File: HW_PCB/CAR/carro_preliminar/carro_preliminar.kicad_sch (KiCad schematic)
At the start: 44 parts, among them IC1 TB6612FNG, J1 V_Battery, J2 STLINK, J3 Motores, J4 BATTLEDS, J5 UART, J6 Servo_Motor, J7 NRF24L01, SW1 SW_DPST_x2, U1 STM32F103C8Tx, U2 AMS1117-3.3, U3 AMS1117-3.3, U5 AMS1117-5.0, Y1 8MHz

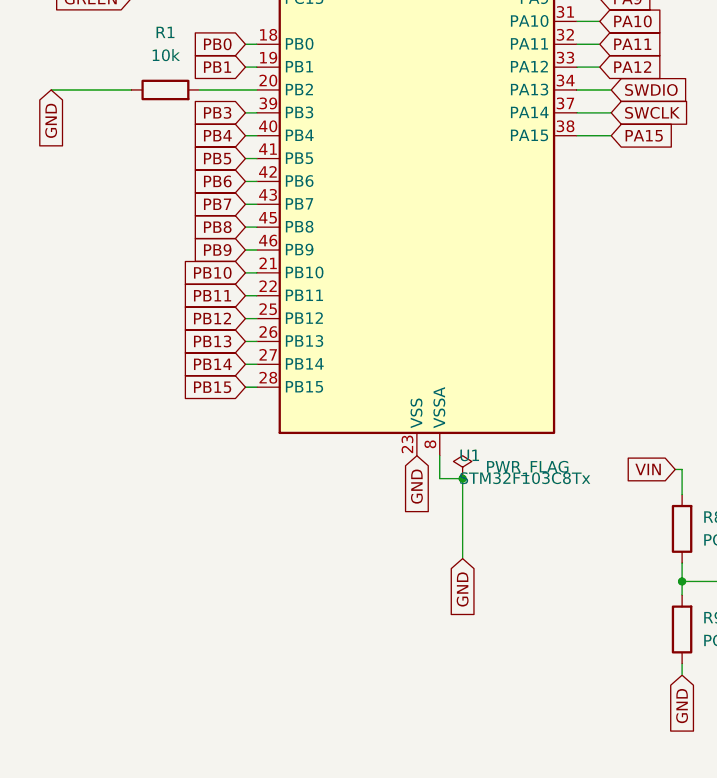
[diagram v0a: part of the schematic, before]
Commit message: PCBCAR FULL
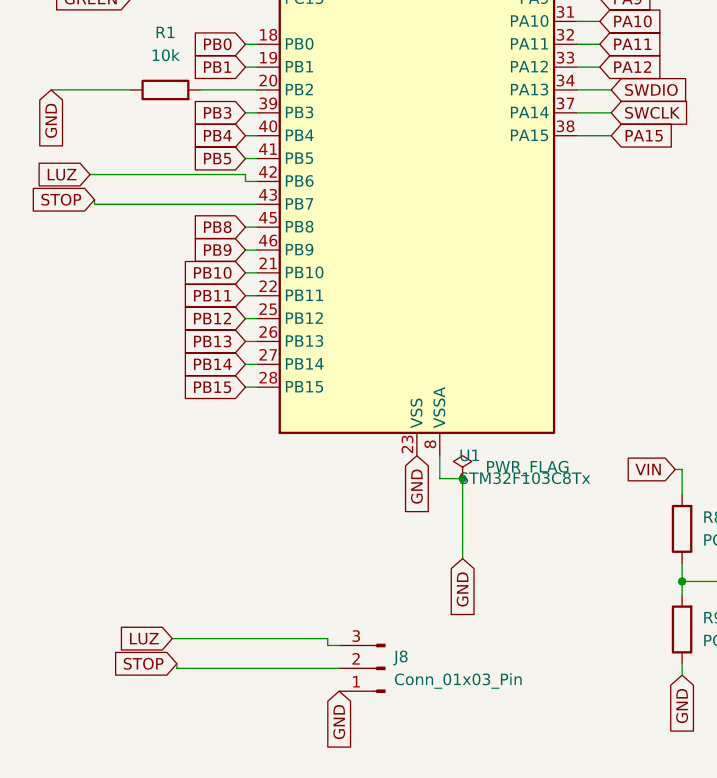
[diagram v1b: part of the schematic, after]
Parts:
- added J8: Conn_01x03_Pin, Connector_PinHeader_2.54mm:PinHeader_1x03_P2.54mm_Vertical, symbol Connector:Conn_01x03_Pin
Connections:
- net GND: now also J8.1 (Pin_1)
- net PB6 renamed LUZ
- net LUZ: now also J8.3 (Pin_3)
- net PB7 renamed STOP
- net STOP: now also J8.2 (Pin_2)
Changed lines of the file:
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@@
 	(wire
 		(pts
+			(xy 47.244 184.15) (xy 47.244 184.912)
+		)
+		(stroke
+			(width 0)
+			(type default)
+		)
+	)
+	(wire
+		(pts
 			(xy 161.29 71.12) (xy 161.29 90.17)
 		)
@@
 	(wire
 		(pts
-			(xy 38.1 135.89) (xy 39.37 135.89)
-		)
-		(stroke
-			(width 0)
-			(type default)
-		)
-	)
-	(wire
-		(pts
 			(xy 161.29 119.38) (xy 162.56 119.38)
 		)
@@
 	(wire
 		(pts
+			(xy 21.336 135.382) (xy 21.336 135.89)
+		)
+		(stroke
+			(width 0)
+			(type default)
+		)
+	)
+	(wire
+		(pts
 			(xy 229.108 138.684) (xy 242.062 138.684)
 		)
@@
 	(wire
 		(pts
+			(xy 20.828 132.588) (xy 38.1 132.588)
+		)
+		(stroke
+			(width 0)
+			(type default)
+		)
+	)
+	(wire
+		(pts
 			(xy 74.93 107.95) (xy 77.47 107.95)
 		)
@@
 	(wire
 		(pts
+			(xy 29.972 184.15) (xy 47.244 184.15)
+		)
+		(stroke
+			(width 0)
+			(type default)
+		)
+	)
+	(wire
+		(pts
 			(xy 38.1 133.35) (xy 39.37 133.35)
 		)
@@
 	(wire
 		(pts
+			(xy 21.336 135.89) (xy 39.37 135.89)
+		)
+		(stroke
+			(width 0)
+			(type default)
+		)
+	)
+	(wire
+		(pts
 			(xy 172.72 77.47) (xy 175.26 77.47)
 		)
@@
 	(wire
 		(pts
+			(xy 38.1 132.588) (xy 38.1 133.35)
+		)
+		(stroke
+			(width 0)
+			(type default)
+		)
+	)
+	(wire
+		(pts
 			(xy 91.694 177.8) (xy 86.614 177.8)
 		)
@@
 	(wire
 		(pts
+			(xy 30.48 187.452) (xy 48.514 187.452)
+		)
+		(stroke
+			(width 0)
+			(type default)
+		)
+	)
+	(wire
+		(pts
 			(xy 214.63 74.93) (xy 214.63 97.79)
 		)
@@
 	(wire
 		(pts
+			(xy 30.48 186.944) (xy 30.48 187.452)
+		)
+		(stroke
+			(width 0)
+			(type default)
+		)
+	)
+	(wire
+		(pts
 			(xy 191.262 147.32) (xy 191.262 152.908)
 		)
@@
 	(wire
 		(pts
+			(xy 47.244 184.912) (xy 48.514 184.912)
+		)
+		(stroke
+			(width 0)
+			(type default)
+		)
+	)
+	(wire
+		(pts
 			(xy 57.15 78.74) (xy 57.15 82.55)
 		)
@@
 		)
 	)
+	(global_label "GND"
+		(shape input)
+		(at 48.514 189.992 270)
+		(fields_autoplaced yes)
+		(effects
+			(font
+				(size 1.27 1.27)
+			)
+			(justify right)
+		)
+		(property "Intersheetrefs" "${INTERSHEET_REFS}"
+			(at 48.514 196.8477 90)
+			(effects
+				(font
+					(size 1.27 1.27)
+				)
+				(justify right)
+				(hide yes)
+			)
+		)
+	)
 	(global_label "PA6"
 		(shape input)
@@
 		)
 	)
+	(global_label "STOP"
+		(shape input)
+		(at 21.336 135.382 180)
+		(fields_autoplaced yes)
+		(effects
+			(font
+				(size 1.27 1.27)
+			)
+			(justify right)
+		)
+		(property "Intersheetrefs" "${INTERSHEET_REFS}"
+			(at 13.5732 135.382 0)
+			(effects
+				(font
+					(size 1.27 1.27)
+				)
+				(justify right)
+				(hide yes)
+			)
+		)
+	)
 	(global_label "GND"
 		(shape input)
@@
 		)
 	)
-	(global_label "PB7"
-		(shape input)
-		(at 38.1 135.89 180)
-		(fields_autoplaced yes)
-		(effects
-			(font
-				(size 1.27 1.27)
-			)
-			(justify right)
-		)
-		(property "Intersheetrefs" "${INTERSHEET_REFS}"
-			(at 31.3653 135.89 0)
-			(effects
-				(font
-					(size 1.27 1.27)
-				)
-				(justify right)
-				(hide yes)
-			)
-		)
-	)
 	(global_label "GND"
 		(shape input)
@@
 		)
 	)
+	(global_label "STOP"
+		(shape input)
+		(at 30.48 186.944 180)
+		(fields_autoplaced yes)
+		(effects
+			(font
+				(size 1.27 1.27)
+			)
+			(justify right)
+		)
+		(property "Intersheetrefs" "${INTERSHEET_REFS}"
+			(at 22.7172 186.944 0)
+			(effects
+				(font
+					(size 1.27 1.27)
+				)
+				(justify right)
+				(hide yes)
+			)
+		)
+	)
 	(global_label "PA0"
 		(shape input)
@@
 		)
 	)
+	(global_label "LUZ"
+		(shape input)
+		(at 29.972 184.15 180)
+		(fields_autoplaced yes)
+		(effects
+			(font
+				(size 1.27 1.27)
+			)
+			(justify right)
+		)
+		(property "Intersheetrefs" "${INTERSHEET_REFS}"
+			(at 23.4187 184.15 0)
+			(effects
+				(font
+					(size 1.27 1.27)
+				)
+				(justify right)
+				(hide yes)
+			)
+		)
+	)
 	(global_label "GREEN"
 		(shape input)
@@
 		)
 	)
-	(global_label "PB6"
-		(shape input)
-		(at 38.1 133.35 180)
-		(fields_autoplaced yes)
-		(effects
-			(font
-				(size 1.27 1.27)
-			)
-			(justify right)
-		)
-		(property "Intersheetrefs" "${INTERSHEET_REFS}"
-			(at 31.3653 133.35 0)
-			(effects
-				(font
-					(size 1.27 1.27)
-				)
-				(justify right)
-				(hide yes)
-			)
-		)
-	)
 	(global_label "PB0"
 		(shape input)
@@
 		)
 	)
+	(global_label "LUZ"
+		(shape input)
+		(at 20.828 132.588 180)
+		(fields_autoplaced yes)
+		(effects
+			(font
+				(size 1.27 1.27)
+			)
+			(justify right)
+		)
+		(property "Intersheetrefs" "${INTERSHEET_REFS}"
+			(at 14.2747 132.588 0)
+			(effects
+				(font
+					(size 1.27 1.27)
+				)
+				(justify right)
+				(hide yes)
+			)
+		)
+	)
 	(global_label "VCC"
 		(shape input)
@@
 					(unit 1)
 				)
+			)
+		)
+	)
+	(symbol
+		(lib_id "Connector:Conn_01x03_Pin")
+		(at 53.594 187.452 180)
+		(unit 1)
+		(exclude_from_sim no)
+		(in_bom yes)
+		(on_board yes)
+		(dnp no)
+		(fields_autoplaced yes)
+		(property "Reference" "J8"
+			(at 54.61 186.1819 0)
+			(effects
+				(font
+					(size 1.27 1.27)
+				)
+				(justify right)
+			)
+		)
+		(property "Value" "Conn_01x03_Pin"
+			(at 54.61 188.7219 0)
+			(effects
+				(font
+					(size 1.27 1.27)
+				)
+				(justify right)
+			)
+		)
+		(property "Footprint" "Connector_PinHeader_2.54mm:PinHeader_1x03_P2.54mm_Vertical"
+			(at 53.594 187.452 0)
+			(effects
+				(font
+					(size 1.27 1.27)
+				)
+				(hide yes)
+			)
+		)
+		(property "Datasheet" "~"
+			(at 53.594 187.452 0)
+			(effects
+				(font
+					(size 1.27 1.27)
+				)
+				(hide yes)
+			)
+		)
+		(property "Description" "Generic connector, single row, 01x03, script generated"
+			(at 53.594 187.452 0)
+			(effects
+				(font
+					(size 1.27 1.27)
+				)
+				(hide yes)
+			)
+		)
+		(pin "2"
+		)
+		(pin "1"
+		)
+		(pin "3"
+		)
+		(instances
+			(project ""
+				(path "/b44e6fd1-366d-4904-8da1-e136aff2ec70"
+					(reference "J8")
+					(unit 1)
+				)
